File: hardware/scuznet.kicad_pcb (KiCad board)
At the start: 2 copper layers, 100 x 79.5 mm, 96 parts, among them J1 SCSI, J2 Barrel_Jack_2P, J3 RJ45-TRANSFO, J4 Micro_SD_Card, J5 PDI, J6 HS, J7 HS, U1 ATXMEGA128A3U, U10 LM1117-ADJ, U2 74LVTH126, U3 74LVTH126, U4 74LVTH126, U5 74LVTH126, U6 74LVC14, U7 74LVTH574, U8 ENC28J60-I/SP, U9 MCP1826S, Y1 25MHz

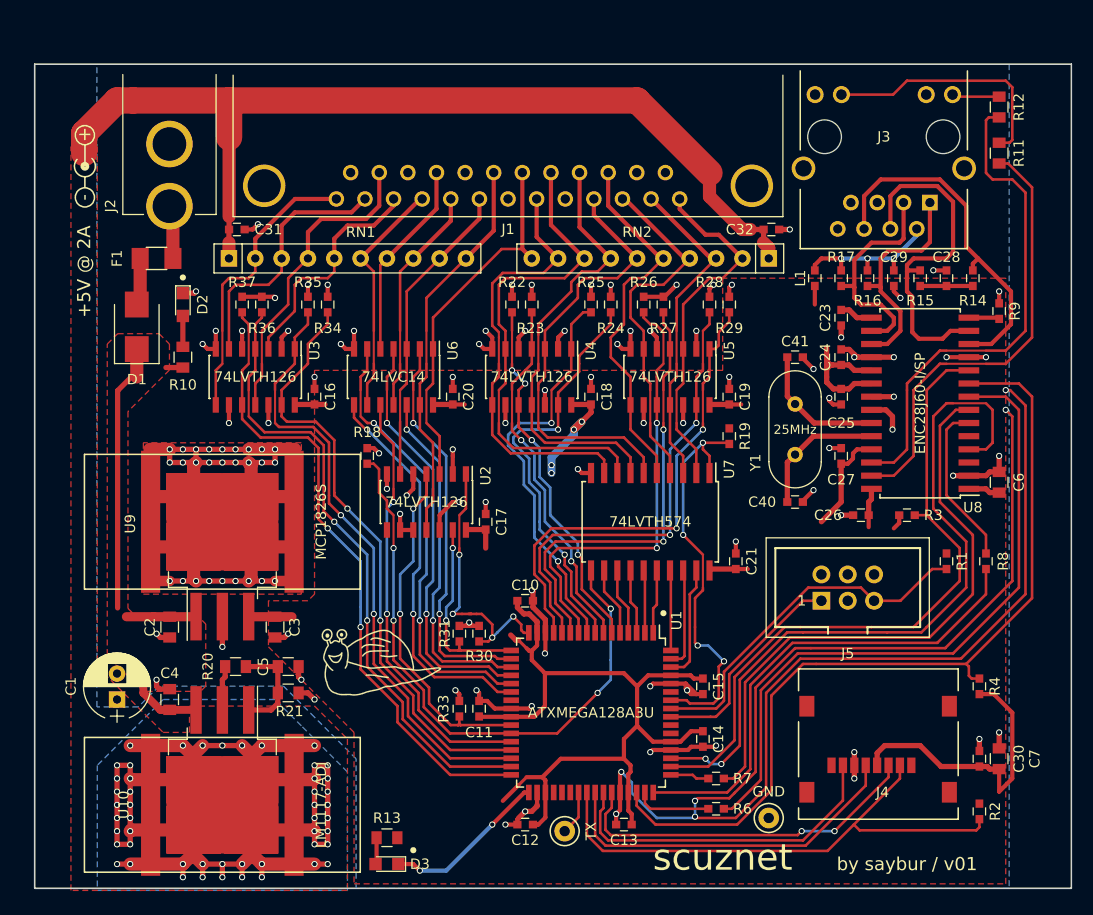
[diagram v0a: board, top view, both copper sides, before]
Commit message: Hardware revision 2.
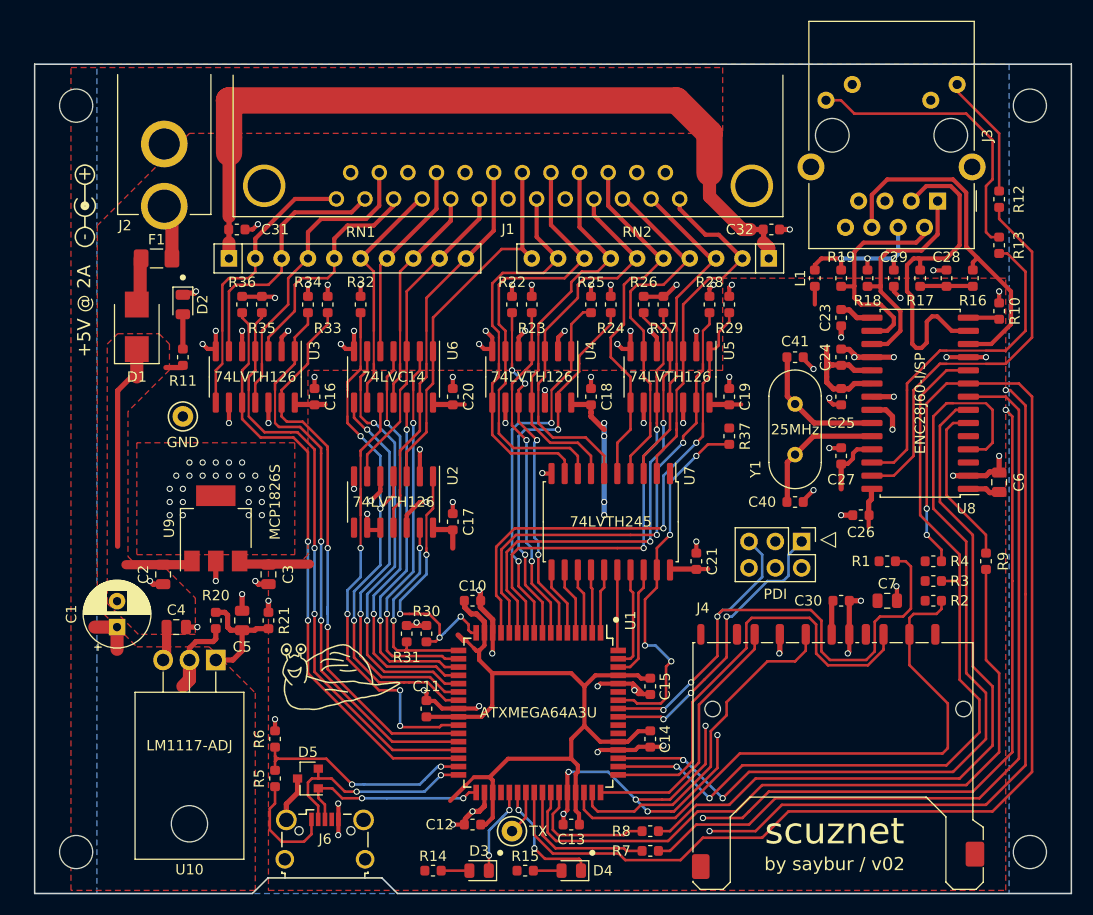
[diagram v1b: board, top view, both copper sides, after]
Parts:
- removed J7: HS, Heatsinks:Heatsink_AAVID_573300D00010G_TO-263
- removed the R10 at (74.3, 88.3)
- removed the R18 at (92.1, 97.8)
- removed the R19 at (127.0, 95.9)
- added D4: LED, LED_SMD:LED_0805_2012Metric, F.Cu at (111.8, 137.8)
- added D5: SP0502BAHT, Package_TO_SOT_SMD:SOT-23, F.Cu at (86.4, 128.9)
- added R12: 330, Resistor_SMD:R_0603_1608Metric, F.Cu at (153.0, 73.0)
- added R15: 165, Resistor_SMD:R_0603_1608Metric, F.Cu at (107.3, 137.8)
- added R37: 3K3, Resistor_SMD:R_0603_1608Metric, F.Cu at (127.0, 95.9)
- added R5: 10K, Resistor_SMD:R_0603_1608Metric, F.Cu at (83.2, 128.9)
- added R6: 10K, Resistor_SMD:R_0603_1608Metric, F.Cu at (83.2, 125.1)
- added REF**: MountingHole_3.2mm_M3, MountingHole:MountingHole_3.2mm_M3, F.Cu at (156.0, 136.0)
- added REF**: MountingHole_3.2mm_M3, MountingHole:MountingHole_3.2mm_M3, F.Cu at (64.0, 136.0)
- added REF**: MountingHole_3.2mm_M3, MountingHole:MountingHole_3.2mm_M3, F.Cu at (64.0, 64.0)
- added REF**: MountingHole_3.2mm_M3, MountingHole:MountingHole_3.2mm_M3, F.Cu at (156.0, 64.0)
- C1: footprint Capacitors_THT:CP_Radial_D6.3mm_P2.50mm -> Capacitor_THT:CP_Radial_D6.3mm_P2.50mm
- C10, C11, C12, C13, C14, C15, C16, C17, C18, C19, C20, C21, C23, C24, C25, C26, C27, C28, C29, C30, C31, C32, C40, C41, L1: footprint Capacitors_SMD:C_0603 -> Capacitor_SMD:C_0603_1608Metric
- C2, C3, C4, C5, C6, C7: footprint Capacitors_SMD:C_0805 -> Capacitor_SMD:C_0805_2012Metric
- D1: footprint Diodes_SMD:D_SMB -> Diode_SMD:D_SMB
- D2, D3: footprint LEDs:LED_0805 -> LED_SMD:LED_0805_2012Metric
- F1: footprint Fuse_Holders_and_Fuses:Fuse_SMD1206_Wave -> Fuse:Fuse_1206_3216Metric_Pad1.42x1.75mm_HandSolder
- J3: footprint scuznet:SI-60062-F -> Connector_RJ:RJ45_Amphenol_RJMG1BD3B8K1ANR
- J4: value Micro_SD_Card -> SD_Card; footprint scuznet:0472192001 -> Connector_Card:SD_Kyocera_145638009211859+
- J5: footprint Connectors:IDC_Header_Straight_6pins -> Connector_PinHeader_2.54mm:PinHeader_2x03_P2.54mm_Vertical
- J6: value HS -> USB_B_Micro; footprint Heatsinks:Heatsink_AAVID_573300D00010G_TO-263 -> Connector_USB:USB_Micro-B_Wuerth_629105150521_CircularHoles
- R1, R2, R22, R23, R24, R25, R26, R27, R28, R29, R3, R30, R31, R4: footprint Capacitors_SMD:C_0603 -> Resistor_SMD:R_0603_1608Metric
- R10: renamed from R9; footprint Capacitors_SMD:C_0603 -> Resistor_SMD:R_0603_1608Metric
- R11, R20, R21: footprint Capacitors_SMD:C_0805 -> Resistor_SMD:R_0603_1608Metric
- R13: renamed from R12; footprint Capacitors_SMD:C_0805 -> Resistor_SMD:R_0603_1608Metric
- R14: renamed from R13; footprint Capacitors_SMD:C_0805 -> Resistor_SMD:R_0603_1608Metric
- R16: renamed from R14; footprint Capacitors_SMD:C_0603 -> Resistor_SMD:R_0603_1608Metric
- R17: renamed from R15; footprint Capacitors_SMD:C_0603 -> Resistor_SMD:R_0603_1608Metric
- R18: renamed from R16; footprint Capacitors_SMD:C_0603 -> Resistor_SMD:R_0603_1608Metric
- R19: renamed from R17; footprint Capacitors_SMD:C_0603 -> Resistor_SMD:R_0603_1608Metric
- R32: renamed from R33; footprint Capacitors_SMD:C_0603 -> Resistor_SMD:R_0603_1608Metric
- R33: renamed from R34; footprint Capacitors_SMD:C_0603 -> Resistor_SMD:R_0603_1608Metric
- R34: renamed from R35; footprint Capacitors_SMD:C_0603 -> Resistor_SMD:R_0603_1608Metric
- R35: renamed from R36; footprint Capacitors_SMD:C_0603 -> Resistor_SMD:R_0603_1608Metric
- R36: renamed from R37; footprint Capacitors_SMD:C_0603 -> Resistor_SMD:R_0603_1608Metric
- R7: renamed from R6; footprint Capacitors_SMD:C_0603 -> Resistor_SMD:R_0603_1608Metric
- R8: renamed from R7; footprint Capacitors_SMD:C_0603 -> Resistor_SMD:R_0603_1608Metric
- R9: renamed from R8; footprint Capacitors_SMD:C_0603 -> Resistor_SMD:R_0603_1608Metric
- RN1, RN2: footprint Resistors_THT:R_Array_SIP10 -> Resistor_THT:R_Array_SIP10
- TP1, TP2: footprint Connectors_TestPoints:Test_Point_Keystone_5000-5004_Miniature -> TestPoint:TestPoint_Keystone_5000-5004_Miniature
- U1: value ATXMEGA128A3U -> ATXMEGA64A3U; footprint Housings_QFP:TQFP-64_14x14mm_Pitch0.8mm -> Package_QFP:TQFP-64_14x14mm_P0.8mm
- U10: footprint TO_SOT_Packages_SMD:TO-263-3_TabPin2 -> Package_TO_SOT_THT:TO-220F-3_Horizontal_TabDown
- U2, U3, U4, U5, U6: footprint Housings_SOIC:SOIC-14_3.9x8.7mm_Pitch1.27mm -> Package_SO:SOIC-14_3.9x8.7mm_P1.27mm
- U7: value 74LVTH574 -> 74LVTH245; footprint Housings_SOIC:SOIC-20W_7.5x12.8mm_Pitch1.27mm -> Package_SO:SOIC-20W_7.5x12.8mm_P1.27mm
- U8: footprint Housings_SOIC:SOIC-28W_7.5x17.9mm_Pitch1.27mm -> Package_SO:SOIC-28W_7.5x17.9mm_P1.27mm
- U9: footprint TO_SOT_Packages_SMD:TO-263-3_TabPin2 -> Package_TO_SOT_SMD:SOT-223-3_TabPin2
- Y1: footprint Crystals:Crystal_HC49-U_Vertical -> Crystal:Crystal_HC49-4H_Vertical
- moved R11 81.2 mm to (74.3, 88.3), turned to 270 degrees
- moved TP2 68.5 mm to (74.3, 94.0)
- moved R32 40.1 mm to (91.4, 83.2)
- moved J6 32.2 mm to (88.0, 134.8)
- moved R2 20.8 mm to (146.7, 111.8), turned to 0 degrees
- moved C30 20.3 mm to (137.8, 111.8), turned to 0 degrees
- moved C7 18.7 mm to (142.2, 111.8), turned to 0 degrees
- moved R13 13.3 mm to (153.0, 77.5)
- moved R4 12.9 mm to (146.7, 108.0), turned to 180 degrees
- moved U10 10.6 mm to (77.5, 117.5), turned to 180 degrees
- moved D3 8.91 mm to (102.9, 137.8)
- moved R8 8.13 mm to (119.4, 134.0)
- moved R7 7.54 mm to (119.4, 135.9)
- moved R21 7.24 mm to (82.5, 113.7), turned to 90 degrees
- moved C4 7.01 mm to (73.7, 114.3), turned to 0 degrees
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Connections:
- D3 pad 1: /LED -> /LED1
- J4 pad 1: Net-(J4-Pad1) -> /~SD_CS
- J4 pad 2: /~SD_CS -> /SD_MOSI
- J4 pad 3: /SD_MOSI -> GND
- J6 pad 1: GND -> Net-(J6-Pad1)
- R11 pad 1: Net-(R11-Pad1) -> Net-(D2-Pad2)
- R11 pad 2: /LEDA -> +5V
- R7 pad 1: Net-(R6-Pad1) -> Net-(R7-Pad1)
- R8 pad 1: Net-(R7-Pad1) -> Net-(R8-Pad1)
- U1 pad 23: Net-(U1-Pad23) -> /TBSY
- U1 pad 26: /TBSY -> /RACK
- U1 pad 27: /DCLK -> /TCD
- U1 pad 28: /RACK -> /TIO
- U1 pad 29: /TCD -> /TMSG
- U1 pad 30: /TIO -> /TREQ
- U1 pad 31: /TMSG -> Net-(R5-Pad1)
- U1 pad 32: /TREQ -> Net-(D5-Pad2)
- U1 pad 33: /LED -> Net-(D5-Pad1)
- U1 pad 37: Net-(U1-Pad37) -> /LED1
- U1 pad 38: Net-(U1-Pad38) -> /LED2
- U1 pad 40: /~SD_CS -> /~E_CS
- U1 pad 41: /SD_SCK -> Net-(R7-Pad1)
- U1 pad 42: /SD_MISO -> /E_MISO
- U1 pad 43: /SD_MOSI -> Net-(R8-Pad1)
- U1 pad 46: /~E_CS -> /~SD_CS
- U1 pad 47: Net-(R6-Pad1) -> /SD_SCK
- U1 pad 48: /E_MISO -> /SD_MISO
- U1 pad 49: Net-(R7-Pad1) -> /SD_MOSI
- U7 pad 1: /~DOE -> VCC
- U7 pad 11: /DCLK -> /RDB0
- U7 pad 12: /RDB0 -> /RDB1
- U7 pad 13: /RDB1 -> /RDB2
- U7 pad 14: /RDB2 -> /RDB3
- U7 pad 15: /RDB3 -> /RDB4
- U7 pad 16: /RDB4 -> /RDB5
- U7 pad 17: /RDB5 -> /RDB6
- U7 pad 18: /RDB6 -> /RDB7
- U7 pad 19: /RDB7 -> /~DOE
- U8 pad 27: Net-(R11-Pad1) -> Net-(R12-Pad1)
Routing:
- net VBUS: track 224.3 -> 92.2 mm, vias 49 -> 0
- net /DCLK: track 58.7 -> 0.00 mm, vias 4 -> 0
- net Net-(R11-Pad1): track 43.3 -> 0.00 mm
- net GND: track 391.3 -> 349.3 mm, vias 118 -> 121
- net Net-(R12-Pad1): track 0.00 -> 38.6 mm
- net /~E_CS: track 83.0 -> 120.1 mm, vias 0 -> 2
- net VCC: track 174.0 -> 147.5 mm
- net /LEDB: track 4.58 -> 28.3 mm
- net Net-(J5-Pad5): track 34.9 -> 57.8 mm, vias 0 -> 3
- net /E_MISO: track 47.2 -> 69.6 mm
- net Net-(R5-Pad1): track 0.00 -> 22.1 mm, vias 0 -> 2
- net Net-(D5-Pad2): track 0.00 -> 20.8 mm, vias 0 -> 2
- net Net-(D5-Pad1): track 0.00 -> 19.1 mm, vias 0 -> 2
- net /TBSY: track 34.2 -> 51.8 mm, vias 2 -> 3
- net /~E_RST: track 64.6 -> 81.0 mm, vias 0 -> 2
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- removed copper zone on B.Cu, net VBUS
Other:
- board size 100 x 79.5 mm -> 100 x 80 mm
- board text added: "by saybur / v02"
- board text added: "▷"
- board text removed: "by saybur / v01"

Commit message: Add files via upload
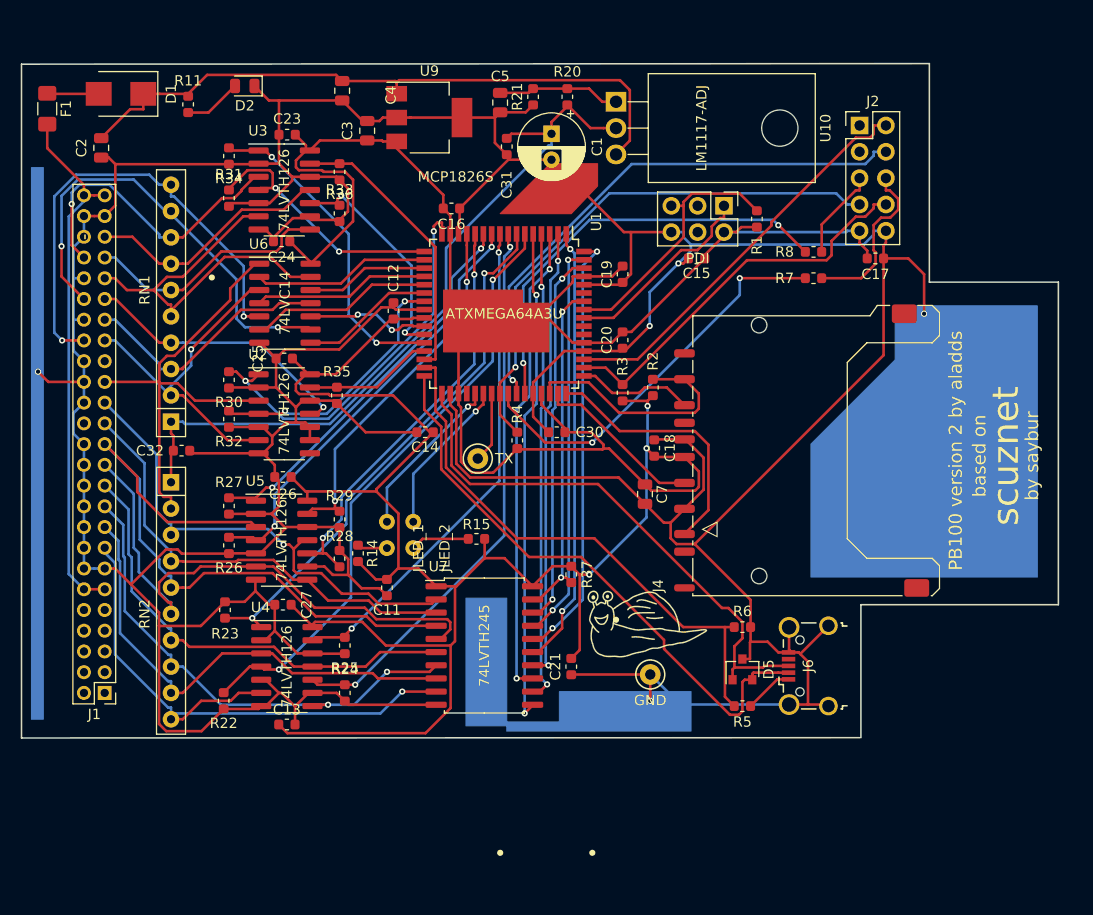
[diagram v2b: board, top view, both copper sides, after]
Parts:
- removed C10, C28, C29: 100nF, Capacitor_SMD:C_0603_1608Metric
- removed C40, C41: 27pF, Capacitor_SMD:C_0603_1608Metric
- removed C6: 10uF, Capacitor_SMD:C_0805_2012Metric
- removed D3, D4: LED, LED_SMD:LED_0805_2012Metric
- removed J3: RJ45-TRANSFO, Connector_RJ:RJ45_Amphenol_RJMG1BD3B8K1ANR
- removed L1: Ferrite_Bead, Capacitor_SMD:C_0603_1608Metric
- removed R10: 2K32, Resistor_SMD:R_0603_1608Metric
- removed R12, R13: 330, Resistor_SMD:R_0603_1608Metric
- removed R16, R17, R18, R19: 49.9, Resistor_SMD:R_0603_1608Metric
- removed R9: 22, Resistor_SMD:R_0603_1608Metric
- removed REF** (x4): MountingHole_3.2mm_M3, MountingHole:MountingHole_3.2mm_M3
- removed REF**: Symbol_Barrel_Polarity, Symbols:Symbol_Barrel_Polarity
- removed U8: ENC28J60-I/SP, Package_SO:SOIC-28W_7.5x17.9mm_P1.27mm
- removed Y1: 25MHz, Crystal:Crystal_HC49-4H_Vertical
- added JLED_1: Conn_01x02, scuznet:2pin, F.Cu at (96.5, 106.7)
- added JLED_2: Conn_01x02, scuznet:2pin, F.Cu at (99.1, 106.7)
- J1: value SCSI -> 50PinSCSI; footprint scuznet:D25S13A -> Connector_PinHeader_2.00mm:PinHeader_2x25_P2.00mm_Vertical
- J2: value Barrel_Jack_2P -> Conn_02x05_Odd_Even_SPI; footprint scuznet:PJ-037A -> Connector_PinHeader_2.54mm:PinHeader_2x05_P2.54mm_Vertical
- moved J2 67.3 mm to (139.6, 65.9), turned to 0 degrees
- moved U10 66.3 mm to (116.1, 63.6), turned to 270 degrees
- moved C1 63.4 mm to (109.9, 66.7), turned to 270 degrees
- moved RN2 61.6 mm to (73.2, 100.3), turned to 270 degrees
- moved R20 60.8 mm to (111.4, 63.1)
- moved C32 60.8 mm to (74.2, 97.3)
- moved R8 58.1 mm to (135.1, 78.1)
- moved R7 57.4 mm to (135.1, 80.6)
- moved R21 56.6 mm to (108.1, 63.1), turned to 270 degrees
- moved C23 56.3 mm to (84.4, 66.8), turned to 180 degrees
- moved C26 55.9 mm to (83.9, 99.8)
- moved C5 55.8 mm to (104.9, 63.7), turned to 270 degrees
- moved C27 55.7 mm to (83.9, 112.1), turned to 180 degrees
- moved C24 55.1 mm to (83.8, 77.1), turned to 180 degrees
- moved C4 54.2 mm to (89.7, 62.6), turned to 270 degrees
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- renumbered G*** to G1***
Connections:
- J1 pad 1: /REQ -> Net-(J1-Pad1)
- J1 pad 10: /DB3 -> Net-(J1-Pad10)
- J1 pad 11: /DB5 -> Net-(F1-Pad2)
- J1 pad 12: /DB6 -> Net-(F1-Pad2)
- J1 pad 13: /DB7 -> GND
- J1 pad 15: /CD -> /DB0
- J1 pad 17: /ATN -> /DB1
- J1 pad 19: /SEL -> /DB2
- J1 pad 2: /MSG -> Net-(J1-Pad2)
- J1 pad 20: /DBP -> GND
- J1 pad 21: /DB1 -> /DB3
- J1 pad 22: /DB2 -> GND
- J1 pad 25: Net-(J1-Pad25) -> /DB5
- J1 pad 3: /IO -> Net-(J1-Pad3)
- J1 pad 4: /RST -> Net-(J1-Pad4)
- J1 pad 5: /ACK -> Net-(J1-Pad5)
- J1 pad 6: /BSY -> Net-(J1-Pad6)
- J1 pad 7: GND -> Net-(J1-Pad7)
- J1 pad 8: /DB0 -> Net-(J1-Pad8)
- J1 pad 9: GND -> Net-(J1-Pad9)
- J2 pad 1: Net-(F1-Pad2) -> Net-(J2-Pad1)
- J2 pad 2: GND -> /~E_INT
- R14 pad 1: Net-(D3-Pad2) -> VCC
- R14 pad 2: VCC -> Net-(JLED_1-Pad1)
- R15 pad 1: Net-(D4-Pad2) -> VCC
- R15 pad 2: VCC -> Net-(JLED_2-Pad1)
- RN1 pad 10: /SEL -> /ATN
- RN1 pad 2: /REQ -> /BSY
- RN1 pad 3: /MSG -> /ACK
- RN1 pad 4: /CD -> /MSG
- RN1 pad 5: /IO -> /SEL
- RN1 pad 6: /RST -> /CD
- RN1 pad 7: /ATN -> /REQ
- RN1 pad 8: /ACK -> /IO
- RN1 pad 9: /BSY -> /RST
- RN2 pad 10: /DBP -> /DB0
- RN2 pad 2: /DB7 -> /DBP
- RN2 pad 3: /DB6 -> /DB7
- RN2 pad 4: /DB5 -> /DB6
- RN2 pad 5: /DB4 -> /DB5
- RN2 pad 6: /DB3 -> /DB4
- RN2 pad 7: /DB2 -> /DB3
- RN2 pad 8: /DB1 -> /DB2
- RN2 pad 9: /DB0 -> /DB1
- U2 pad 11: /SEL -> /MSG
- U2 pad 13: /TSEL -> /TMSG
- U3 pad 10: /TREQ -> /TCD
- U3 pad 11: /CD -> /REQ
- U3 pad 13: /TCD -> /TREQ
- U3 pad 4: /TMSG -> /TSEL
- U3 pad 6: /MSG -> /SEL
- U3 pad 8: /REQ -> /CD
- U4 pad 1: /TDB3 -> /TDB1
- U4 pad 10: /TDB0 -> /TDB2
- U4 pad 11: /DB2 -> /DB3
- U4 pad 13: /TDB2 -> /TDB3
- U4 pad 3: /DB3 -> /DB1
- U4 pad 4: /TDB1 -> /TDB0
- U4 pad 6: /DB1 -> /DB0
- U4 pad 8: /DB0 -> /DB2
- U5 pad 1: /TDB7 -> /TDB5
- U5 pad 10: /TDB4 -> /TDB6
- U5 pad 11: /DB6 -> /DB7
- U5 pad 13: /TDB6 -> /TDB7
- U5 pad 3: /DB7 -> /DB5
- U5 pad 4: /TDB5 -> /TDB4
- U5 pad 6: /DB5 -> /DB4
- U5 pad 8: /DB4 -> /DB6
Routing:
- net GND: track 349.3 -> 569.3 mm, vias 121 -> 5
- net VCC: track 147.5 -> 335.6 mm, vias 4 -> 3
- net /~E_CS: track 120.1 -> 52.7 mm, vias 2 -> 1
- net /E_MOSI: track 72.0 -> 8.84 mm
- net /E_SCK: track 77.5 -> 16.3 mm
- net /~E_INT: track 84.9 -> 39.2 mm, vias 2 -> 0
- net Net-(F1-Pad2): track 5.82 -> 51.5 mm
- net /TMSG: track 56.7 -> 12.5 mm, vias 2 -> 0
- net /~E_RST: track 81.0 -> 38.0 mm, vias 2 -> 0
- net /RDB0: track 6.70 -> 48.0 mm, vias 0 -> 2
- net /RDB2: track 6.31 -> 45.7 mm, vias 0 -> 2
- net /RDB1: track 6.50 -> 45.5 mm, vias 0 -> 2
- net Net-(R12-Pad1): track 38.6 -> 0.00 mm
- net /RDB3: track 6.11 -> 43.8 mm, vias 0 -> 2
- net /RDB4: track 6.21 -> 42.7 mm, vias 0 -> 2
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- removed copper zone on F.Cu, net +5V
- removed copper zone on B.Cu, net GND
- removed copper zone on F.Cu, net GND
- removed copper zone on F.Cu, net VBUS
- removed copper zone on F.Cu, net VCC
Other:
- board size 100 x 80 mm -> 100 x 65.1 mm
- board text added: "PB100 version 2 by aladds"
- board text added: "based on"
- board text added: "by saybur"
- board text removed: "+"
- board text removed: "+5V @ 2A"
- board text removed: "by saybur / v02"
